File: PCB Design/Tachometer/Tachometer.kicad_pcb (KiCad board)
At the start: 2 copper layers, 71.1 x 35.6 mm, 1 part, among them U1 STM32F405RGT6

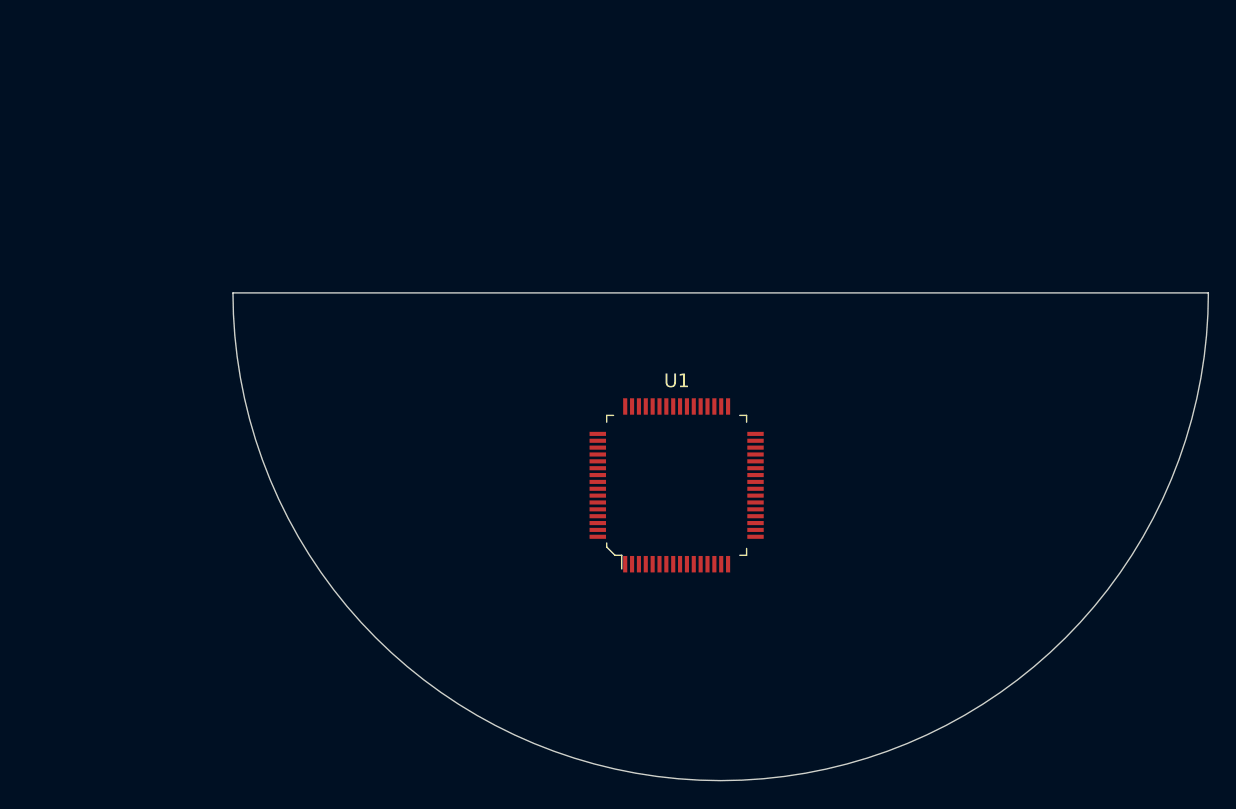
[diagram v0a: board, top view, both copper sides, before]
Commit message: Schematic
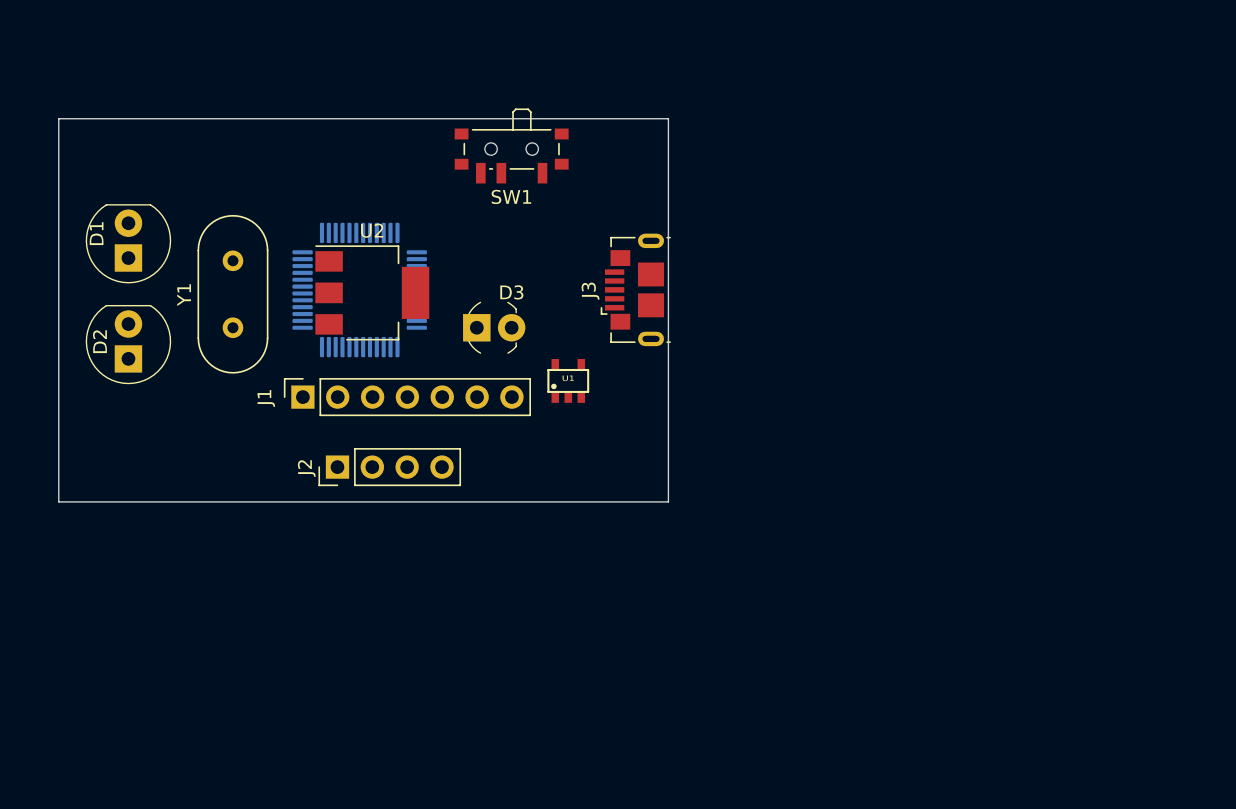
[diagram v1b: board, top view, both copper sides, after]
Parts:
- added D1: IR_Receiver, digikey-footprints:LED_5mm_Radial, F.Cu at (71.1, 55.9)
- added D2: IR_Emitter, digikey-footprints:LED_5mm_Radial, F.Cu at (71.1, 63.2)
- added D3: Indication LED, digikey-footprints:LED_3mm_Radial, F.Cu at (99.1, 63.5)
- added J1: OLED Display, Connector_PinSocket_2.54mm:PinSocket_1x07_P2.54mm_Vertical, F.Cu at (83.8, 68.6)
- added J2: SWD, Connector_PinHeader_2.54mm:PinHeader_1x04_P2.54mm_Vertical, F.Cu at (86.4, 73.7)
- added J3: USB_B_Micro, Connector_USB:USB_Micro-B_GCT_USB3076-30-A, F.Cu at (108.0, 60.7)
- added SW1: SW_SPDT, Button_Switch_SMD:SW_SPDT_PCM12, F.Cu at (99.1, 50.8)
- added U2: AMS1117, Package_TO_SOT_SMD:SOT-223-3_TabPin2, F.Cu at (88.9, 61.0)
- added U3: STM32F103C8Tx, Package_QFP:LQFP-48_7x7mm_P0.5mm, B.Cu at (88.0, 60.8)
- added Y1: Crystal, Crystal:Crystal_HC49-4H_Vertical, F.Cu at (78.7, 63.5)
- U1: value STM32F405RGT6 -> LMV321; footprint digikey-footprints:LQFP-64_10x10mm -> gsg-modules:SOT25
- moved U1 11.0 mm to (103.2, 67.4)
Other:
- board size 71.1 x 35.6 mm -> 44.4 x 27.9 mm

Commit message: Schematic_Update
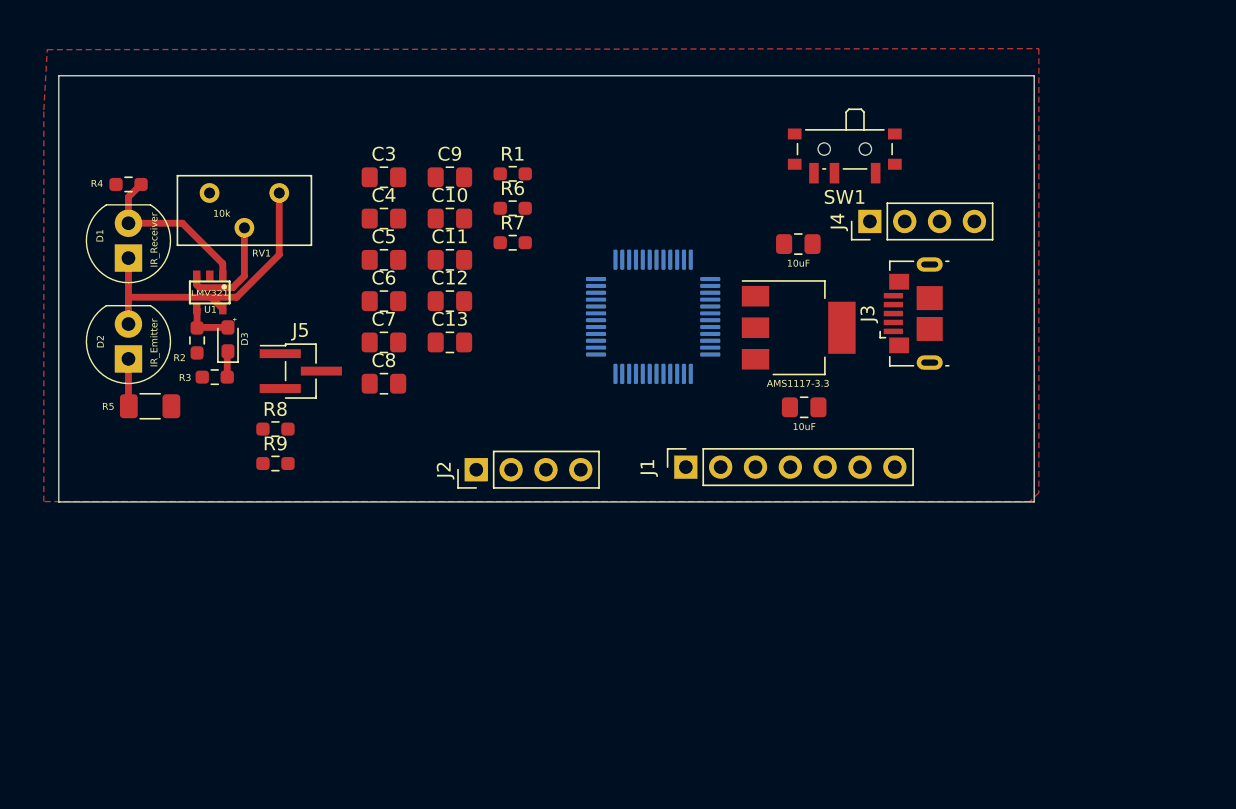
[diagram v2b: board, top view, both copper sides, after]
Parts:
- removed U2: AMS1117, Package_TO_SOT_SMD:SOT-223-3_TabPin2
- removed Y1: Crystal, Crystal:Crystal_HC49-4H_Vertical
- added C1: 10uF, Capacitor_SMD:C_0805_2012Metric_Pad1.18x1.45mm_HandSolder, F.Cu at (120.0, 57.4)
- added C10: 1uF, Capacitor_SMD:C_0805_2012Metric_Pad1.18x1.45mm_HandSolder, F.Cu at (94.6, 55.5)
- added C11: 10uF, Capacitor_SMD:C_0805_2012Metric_Pad1.18x1.45mm_HandSolder, F.Cu at (94.6, 58.5)
- added C12: 100nF, Capacitor_SMD:C_0805_2012Metric_Pad1.18x1.45mm_HandSolder, F.Cu at (94.6, 61.6)
- added C13: 24pF, Capacitor_SMD:C_0805_2012Metric_Pad1.18x1.45mm_HandSolder, F.Cu at (94.6, 64.6)
- added C2: 10uF, Capacitor_SMD:C_0805_2012Metric_Pad1.18x1.45mm_HandSolder, F.Cu at (120.4, 69.3)
- added C3: 24pF, Capacitor_SMD:C_0805_2012Metric_Pad1.18x1.45mm_HandSolder, F.Cu at (89.7, 52.5)
- added C4: 100nF, Capacitor_SMD:C_0805_2012Metric_Pad1.18x1.45mm_HandSolder, F.Cu at (89.7, 55.5)
- added C5: 100nF, Capacitor_SMD:C_0805_2012Metric_Pad1.18x1.45mm_HandSolder, F.Cu at (89.7, 58.5)
- added C6: 100nF, Capacitor_SMD:C_0805_2012Metric_Pad1.18x1.45mm_HandSolder, F.Cu at (89.7, 61.6)
- added C7: 100nF, Capacitor_SMD:C_0805_2012Metric_Pad1.18x1.45mm_HandSolder, F.Cu at (89.7, 64.6)
- added C8: 100nF, Capacitor_SMD:C_0805_2012Metric_Pad1.18x1.45mm_HandSolder, F.Cu at (89.7, 67.6)
- added C9: 100nF, Capacitor_SMD:C_0805_2012Metric_Pad1.18x1.45mm_HandSolder, F.Cu at (94.6, 52.5)
- added J4: UART, Connector_PinHeader_2.54mm:PinHeader_1x04_P2.54mm_Vertical, F.Cu at (125.2, 55.8)
- added J5: Boot0, Connector_PinHeader_1.27mm:PinHeader_1x03_P1.27mm_Vertical_SMD_Pin1Left, F.Cu at (83.7, 66.7)
- added R1: 0R, Resistor_SMD:R_0603_1608Metric_Pad0.98x0.95mm_HandSolder, F.Cu at (99.1, 52.3)
- added R2: 10k, Resistor_SMD:R_0603_1608Metric_Pad0.98x0.95mm_HandSolder, F.Cu at (76.1, 64.4)
- added R3: 1k, Resistor_SMD:R_0603_1608Metric_Pad0.98x0.95mm_HandSolder, F.Cu at (77.4, 67.1)
- added R4: 10k, Resistor_SMD:R_0603_1608Metric_Pad0.98x0.95mm_HandSolder, F.Cu at (71.1, 53.0)
- added R5: 100R, Resistor_SMD:R_1206_3216Metric_Pad1.30x1.75mm_HandSolder, F.Cu at (72.7, 69.2)
- added R6: 10k, Resistor_SMD:R_0603_1608Metric_Pad0.98x0.95mm_HandSolder, F.Cu at (99.1, 54.8)
- added R7: 1.5k, Resistor_SMD:R_0603_1608Metric_Pad0.98x0.95mm_HandSolder, F.Cu at (99.1, 57.3)
- added R8: 1.5k, Resistor_SMD:R_0603_1608Metric_Pad0.98x0.95mm_HandSolder, F.Cu at (81.8, 70.9)
- added R9: 1.5k, Resistor_SMD:R_0603_1608Metric_Pad0.98x0.95mm_HandSolder, F.Cu at (81.8, 73.4)
- added RV1: 10k, Potentiometer_THT:Potentiometer_Bourns_3296Y_Vertical, F.Cu at (82.1, 53.7)
- added U4: AMS1117-3.3, Package_TO_SOT_SMD:SOT-223-3_TabPin2, F.Cu at (120.0, 63.5)
- D3: footprint digikey-footprints:LED_3mm_Radial -> LED_SMD:LED_0603_1608Metric_Pad1.05x0.95mm_HandSolder
- moved J1 28.4 mm to (111.8, 73.7)
- moved U1 26.9 mm to (77.0, 60.9), turned to 180 degrees
- moved SW1 24.3 mm to (123.3, 50.8)
- moved U3 21.5 mm to (109.4, 62.7)
- moved D3 20.7 mm to (78.4, 64.3), turned to 90 degrees
- moved J3 20.4 mm to (128.3, 62.5)
- moved J2 10.1 mm to (96.5, 73.8)
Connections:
- D1 pad 1: unconnected-(D1-K-Pad1) -> /VCC
- D1 pad 2: unconnected-(D1-A-Pad2) -> Net-(D1-A)
- D2 pad 1: unconnected-(D2-K-Pad1) -> Net-(D2-K)
- D2 pad 2: unconnected-(D2-A-Pad2) -> /VCC
- D3 pad 1: unconnected-(D3-K-Pad1) -> Net-(D3-K)
- D3 pad 2: unconnected-(D3-A-Pad2) -> /OP_Out
- J1 pad 1: /GND -> GND
- J2 pad 1: unconnected-(J2-Pin_1-Pad1) -> /VDD
- J2 pad 2: unconnected-(J2-Pin_2-Pad2) -> /SWDIO
- J2 pad 3: unconnected-(J2-Pin_3-Pad3) -> /SWCLK
- J2 pad 4: unconnected-(J2-Pin_4-Pad4) -> GND
- J3 pad 1: unconnected-(J3-VBUS-Pad1) -> /VBUS
- J3 pad 2: unconnected-(J3-D--Pad2) -> /USB_D-
- J3 pad 3: unconnected-(J3-D+-Pad3) -> /USB_D+
- J3 pad 5: unconnected-(J3-GND-Pad5) -> GND
- SW1 pad 1: unconnected-(SW1-A-Pad1) -> /VCC
- SW1 pad 2: unconnected-(SW1-B-Pad2) -> /VBUS
- U1 pad 1: unconnected-(U1-+-Pad1) -> Net-(D1-A)
- U1 pad 2: unconnected-(U1-V--Pad2) -> GND
- U1 pad 3: unconnected-(U1---Pad3) -> Net-(U1--)
- U1 pad 4: unconnected-(U1-Pad4) -> /OP_Out
- U1 pad 5: unconnected-(U1-V+-Pad5) -> /VCC
- U3 pad 1: unconnected-(U3-VBAT-Pad1) -> /VDD
- U3 pad 12: unconnected-(U3-PA2-Pad12) -> /UART_Tx
- U3 pad 13: unconnected-(U3-PA3-Pad13) -> /UART_Rx
- U3 pad 23: Net-(U3-VSS-Pad23) -> GND
- U3 pad 24: unconnected-(U3-VDD-Pad24) -> /VDD
- U3 pad 32: unconnected-(U3-PA11-Pad32) -> /USB_D-
- U3 pad 33: unconnected-(U3-PA12-Pad33) -> /USB_D+
- U3 pad 34: unconnected-(U3-PA13-Pad34) -> /SWDIO
- U3 pad 35: Net-(U3-VSS-Pad23) -> GND
- U3 pad 36: unconnected-(U3-VDD-Pad36) -> /VDD
- U3 pad 37: unconnected-(U3-PA14-Pad37) -> /SWCLK
- U3 pad 42: unconnected-(U3-PB6-Pad42) -> /I2C_SCL
- U3 pad 43: unconnected-(U3-PB7-Pad43) -> /I2C_SDA
- U3 pad 44: unconnected-(U3-BOOT0-Pad44) -> /Boot0
- U3 pad 46: unconnected-(U3-PB9-Pad46) -> /OP_Out
- U3 pad 47: Net-(U3-VSS-Pad23) -> GND
- U3 pad 48: unconnected-(U3-VDD-Pad48) -> /VDD
- U3 pad 5: unconnected-(U3-PD0-Pad5) -> /HSE_IN
- U3 pad 6: unconnected-(U3-PD1-Pad6) -> /HSE_OUT
- U3 pad 7: unconnected-(U3-NRST-Pad7) -> Net-(U3-NRST)
- U3 pad 8: unconnected-(U3-VSSA-Pad8) -> GND
- U3 pad 9: unconnected-(U3-VDDA-Pad9) -> /VDDA
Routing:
- net /VCC: track 0.00 -> 22.8 mm
- net Net-(D1-A): track 0.00 -> 12.2 mm
- net Net-(U1--): track 0.00 -> 8.07 mm
- net /OP_Out: track 0.00 -> 3.66 mm
- net Net-(D2-K): track 0.00 -> 3.47 mm
- net Net-(D3-K): track 0.00 -> 1.90 mm
- added copper zone on F.Cu, net GND
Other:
- board size 44.4 x 27.9 mm -> 71.1 x 31.1 mm
- board text added: "+"

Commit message: PCB_Routed
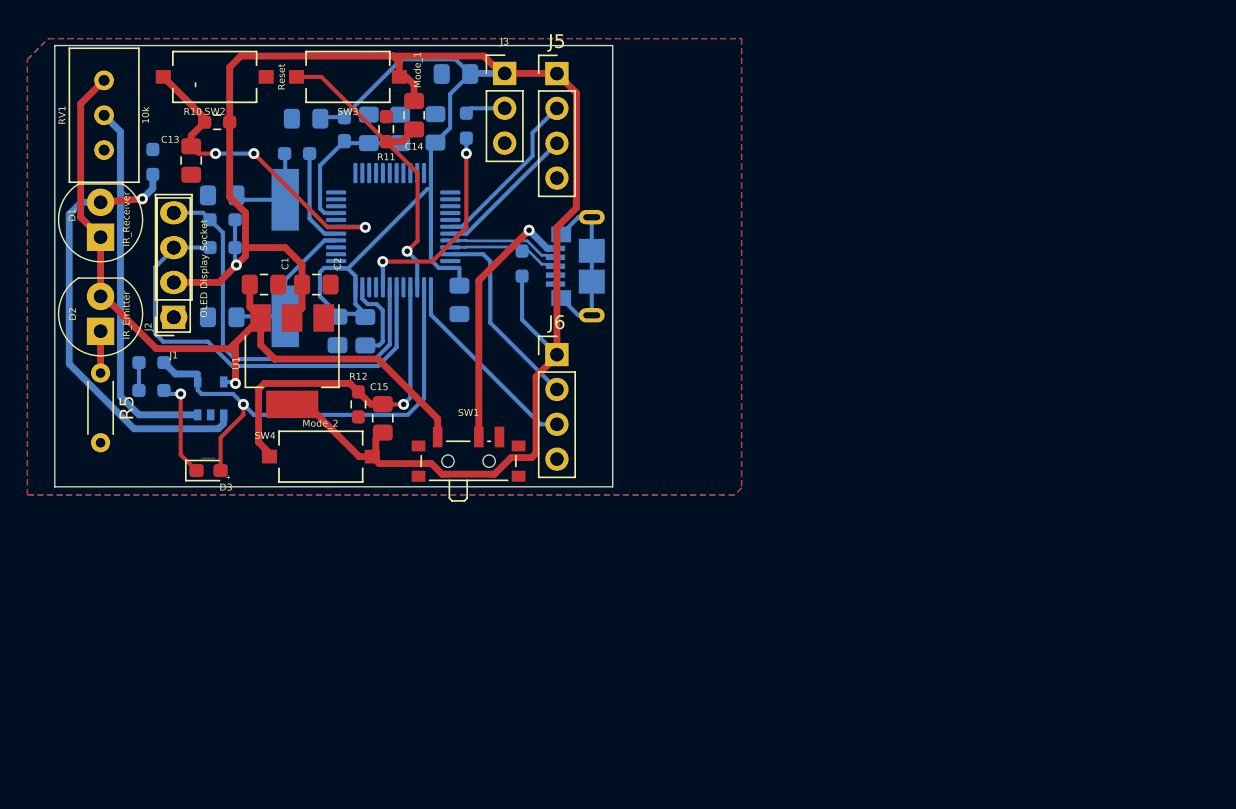
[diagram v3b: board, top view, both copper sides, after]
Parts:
- added C14: 1uF, Capacitor_SMD:C_0805_2012Metric_Pad1.18x1.45mm_HandSolder, F.Cu at (91.9, 48.0)
- added C15: 1uF, Capacitor_SMD:C_0805_2012Metric_Pad1.18x1.45mm_HandSolder, F.Cu at (89.7, 70.1)
- added FB1: 120R, Inductor_SMD:L_0603_1608Metric_Pad1.05x0.95mm_HandSolder, B.Cu at (86.9, 49.0)
- added G***: LOGO, LOGO, B.Cu at (74.7, 45.7)
- added J2: OLED Display, SSD1306:128x64OLED, F.Cu at (85.0, 59.1)
- added R10: 10k, Resistor_SMD:R_0603_1608Metric_Pad0.98x0.95mm_HandSolder, F.Cu at (77.6, 48.5)
- added R11: 10k, Resistor_SMD:R_0603_1608Metric_Pad0.98x0.95mm_HandSolder, F.Cu at (89.9, 49.0)
- added R12: 10k, Resistor_SMD:R_0603_1608Metric_Pad0.98x0.95mm_HandSolder, F.Cu at (87.9, 69.1)
- added Ref**: Val**, SparkFun-Aesthetic:OSHW_Logo_2.5mm, B.Cu at (86.1, 45.5)
- added SW2: Reset, Button_Switch_SMD:SW_TS09-63-25-WT-160-SMT-TR, F.Cu at (77.4, 45.2)
- added SW3: Mode_1, Button_Switch_SMD:SW_TS09-63-25-WT-160-SMT-TR, F.Cu at (87.1, 45.2)
- added SW4: Mode_2, Button_Switch_SMD:SW_TS09-63-25-WT-160-SMT-TR, F.Cu at (85.2, 72.9)
- added Y1: 8MHz_Crystal, Crystal:Crystal_SMD_HC49-SD, B.Cu at (82.5, 58.4)
- C10: renamed from C7; moved to B.Cu
- C11: renamed from C3; value 24pF -> 33pF; moved to B.Cu
- C12: renamed from C13; value 24pF -> 33pF; moved to B.Cu
- C13: renamed from C12; value 100nF -> 1uF
- C3: renamed from C8; moved to B.Cu
- C4: renamed from C10; moved to B.Cu
- C5: renamed from C9; moved to B.Cu
- C6: renamed from C11; moved to B.Cu
- C7: renamed from C4; moved to B.Cu
- C8: renamed from C5; moved to B.Cu
- C9: renamed from C6; moved to B.Cu
- J1: value OLED Display -> OLED Display Socket; footprint Connector_PinSocket_2.54mm:PinSocket_1x07_P2.54mm_Vertical -> Connector_PinSocket_2.54mm:PinSocket_1x04_P2.54mm_Vertical
- J3: renamed from J5; footprint Connector_PinHeader_1.27mm:PinHeader_1x03_P1.27mm_Vertical_SMD_Pin1Left -> Connector_PinHeader_2.54mm:PinHeader_1x03_P2.54mm_Vertical
- J4: renamed from J3; moved to B.Cu
- R1: renamed from R6; moved to B.Cu
- R2: renamed from R4; moved to B.Cu
- R3: renamed from R2; moved to B.Cu
- R4: renamed from R3; moved to B.Cu
- R5: footprint Resistor_SMD:R_1206_3216Metric_Pad1.30x1.75mm_HandSolder -> Resistor_THT:R_Axial_DIN0204_L3.6mm_D1.6mm_P5.08mm_Horizontal
- R6: renamed from R1; moved to B.Cu
- R7, R8, R9: moved to B.Cu
- RV1: footprint Potentiometer_THT:Potentiometer_Bourns_3296Y_Vertical -> Potentiometer_THT:Potentiometer_Bourns_3296W_Vertical
- U2: renamed from U1; moved to B.Cu
- moved C1 39.1 mm to (81.0, 60.4)
- moved J1 38.9 mm to (74.4, 62.7), turned to 180 degrees
- moved U1 37.0 mm to (83.1, 65.9), turned to -90 degrees
- moved C2 36.7 mm to (84.8, 60.4)
- moved SW1 35.2 mm to (95.9, 72.9), turned to 0 degrees
- moved J3 26.3 mm to (98.6, 45.0)
- moved J5 25.2 mm to (102.4, 45.0), turned to 0 degrees
- moved J4 24.9 mm to (103.7, 59.0), turned to -90 degrees
- moved C13 21.5 mm to (75.7, 51.3), turned to 90 degrees
- moved U3 20.0 mm to (90.4, 56.4), turned to 0 degrees
- moved C12 19.8 mm to (78.0, 53.8), turned to 180 degrees
- moved C3 18.6 mm to (88.6, 49.0), turned to 90 degrees
- moved R9 18.2 mm to (78.0, 55.6)
- moved R6 15.8 mm to (83.4, 50.8)
- moved C11 15.6 mm to (78.0, 62.7), turned to 180 degrees
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- renumbered J4 to J5, J2 to J6, U4 to U1
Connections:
- C13 pad 1: Net-(U3-NRST) -> GND
- C13 pad 2: GND -> /Reset
- J1 pad 2: /Vcc -> /VDD
- J1 pad 3: /D0 -> /I2C_SCL
- J1 pad 4: /D1 -> /I2C_SDA
- U3 pad 12: /UART_Tx -> unconnected-(U3-PA2-Pad12)
- U3 pad 13: /UART_Rx -> unconnected-(U3-PA3-Pad13)
- U3 pad 30: unconnected-(U3-PA9-Pad30) -> /UART_Tx
- U3 pad 31: unconnected-(U3-PA10-Pad31) -> /UART_Rx
- U3 pad 38: unconnected-(U3-PA15-Pad38) -> /OP_Out
- U3 pad 39: unconnected-(U3-PB3-Pad39) -> /Mode_1
- U3 pad 40: unconnected-(U3-PB4-Pad40) -> /Mode_2
- U3 pad 46: /OP_Out -> unconnected-(U3-PB9-Pad46)
- U3 pad 7: Net-(U3-NRST) -> /Reset
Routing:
- net /VDD: track 0.00 -> 174.3 mm, vias 0 -> 1
- net /VCC: track 22.8 -> 56.8 mm, vias 0 -> 1
- net /I2C_SCL: track 0.00 -> 32.9 mm
- net /OP_Out: track 3.66 -> 35.3 mm, vias 0 -> 1
- net /I2C_SDA: track 0.00 -> 29.6 mm
- net /Mode_2: track 0.00 -> 25.7 mm, vias 0 -> 1
- net /Reset: track 0.00 -> 24.5 mm, vias 0 -> 3
- net /Mode_1: track 0.00 -> 23.1 mm, vias 0 -> 1
- net Net-(D1-A): track 12.2 -> 32.7 mm, vias 0 -> 1
- net Net-(U2--): track 8.07 -> 27.2 mm
- net /VBUS: track 0.00 -> 19.1 mm, vias 0 -> 1
- net /Boot0: track 0.00 -> 16.0 mm, vias 0 -> 2
- net /SWCLK: track 0.00 -> 14.5 mm
- net /SWDIO: track 0.00 -> 14.5 mm
- net unconnected-(J4-Shield-Pad6): track 0.00 -> 12.6 mm
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- added copper zone on B.Cu, net GND
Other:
- board size 71.1 x 31.1 mm -> 40.7 x 32.2 mm
- board text added: "Made By,"
- board text added: "Open Hardware"
- board text added: "https://github.com/SrikarBharadwajR/Project-Tachometer"
